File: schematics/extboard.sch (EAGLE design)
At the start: 23 parts, among them U1 LTC1257, U2 LTC1257, X1-SD SDBMF, X2-JACK 1503_02

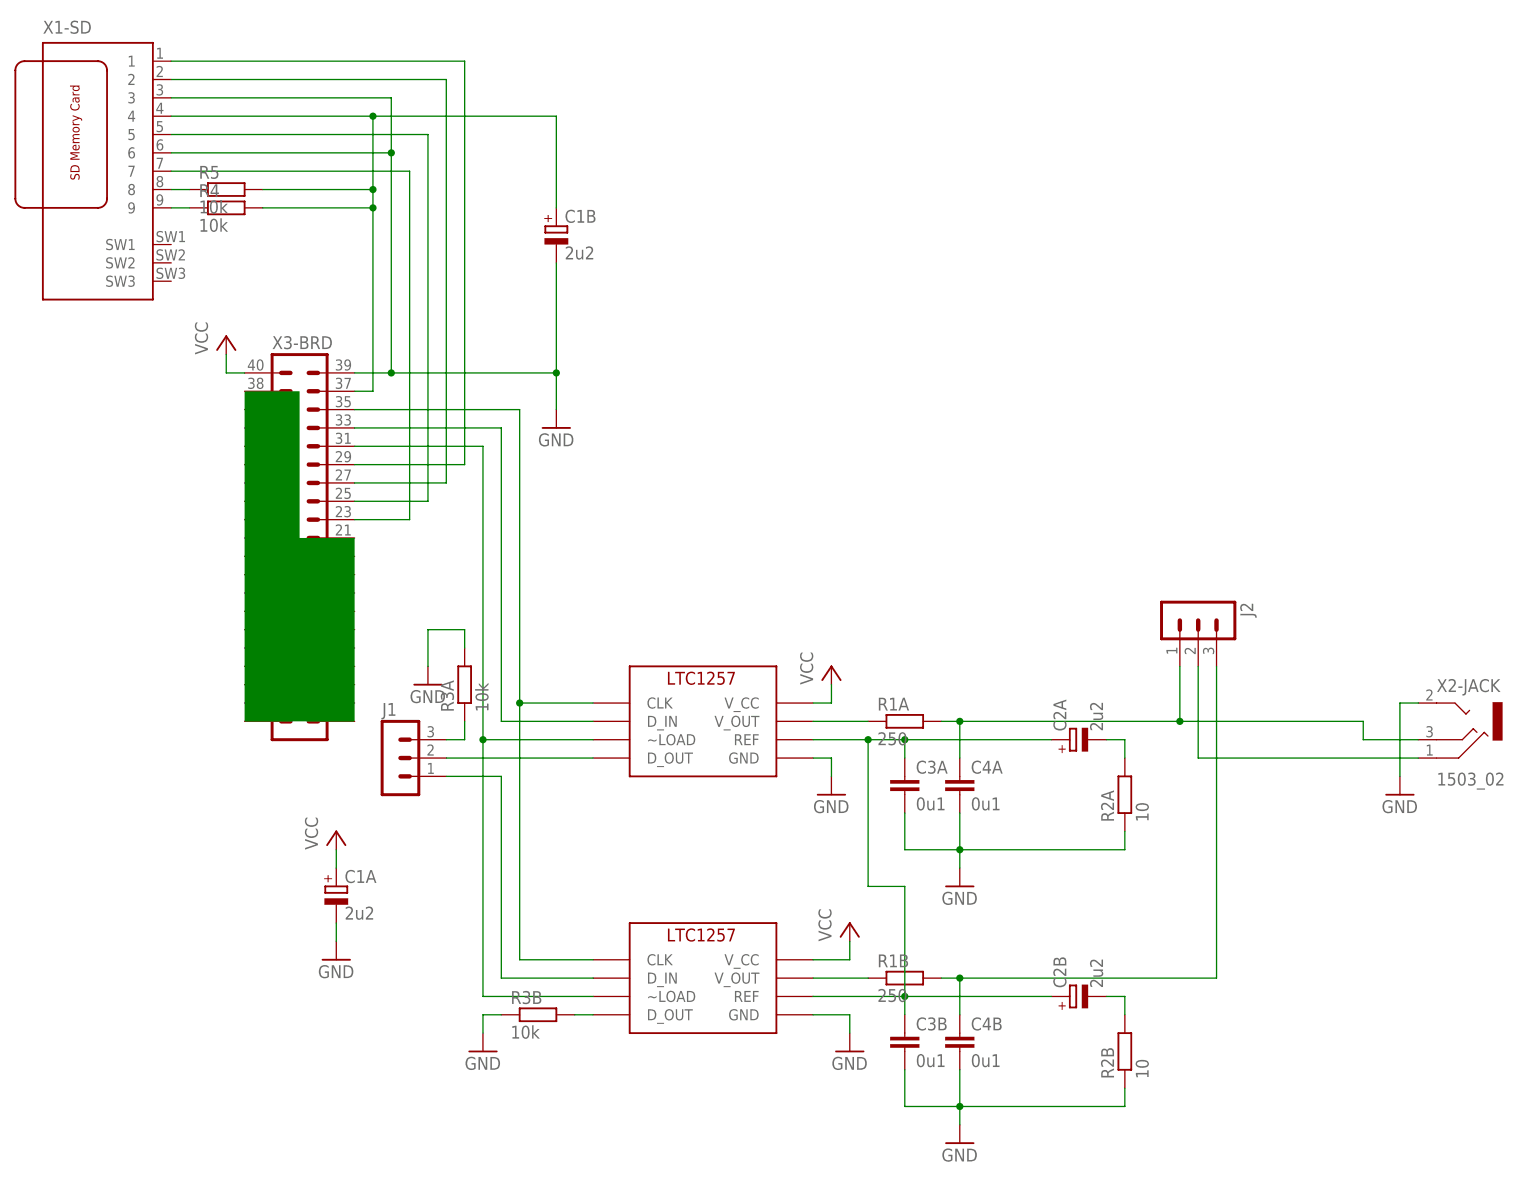
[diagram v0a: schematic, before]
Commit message: schematics: next iteration
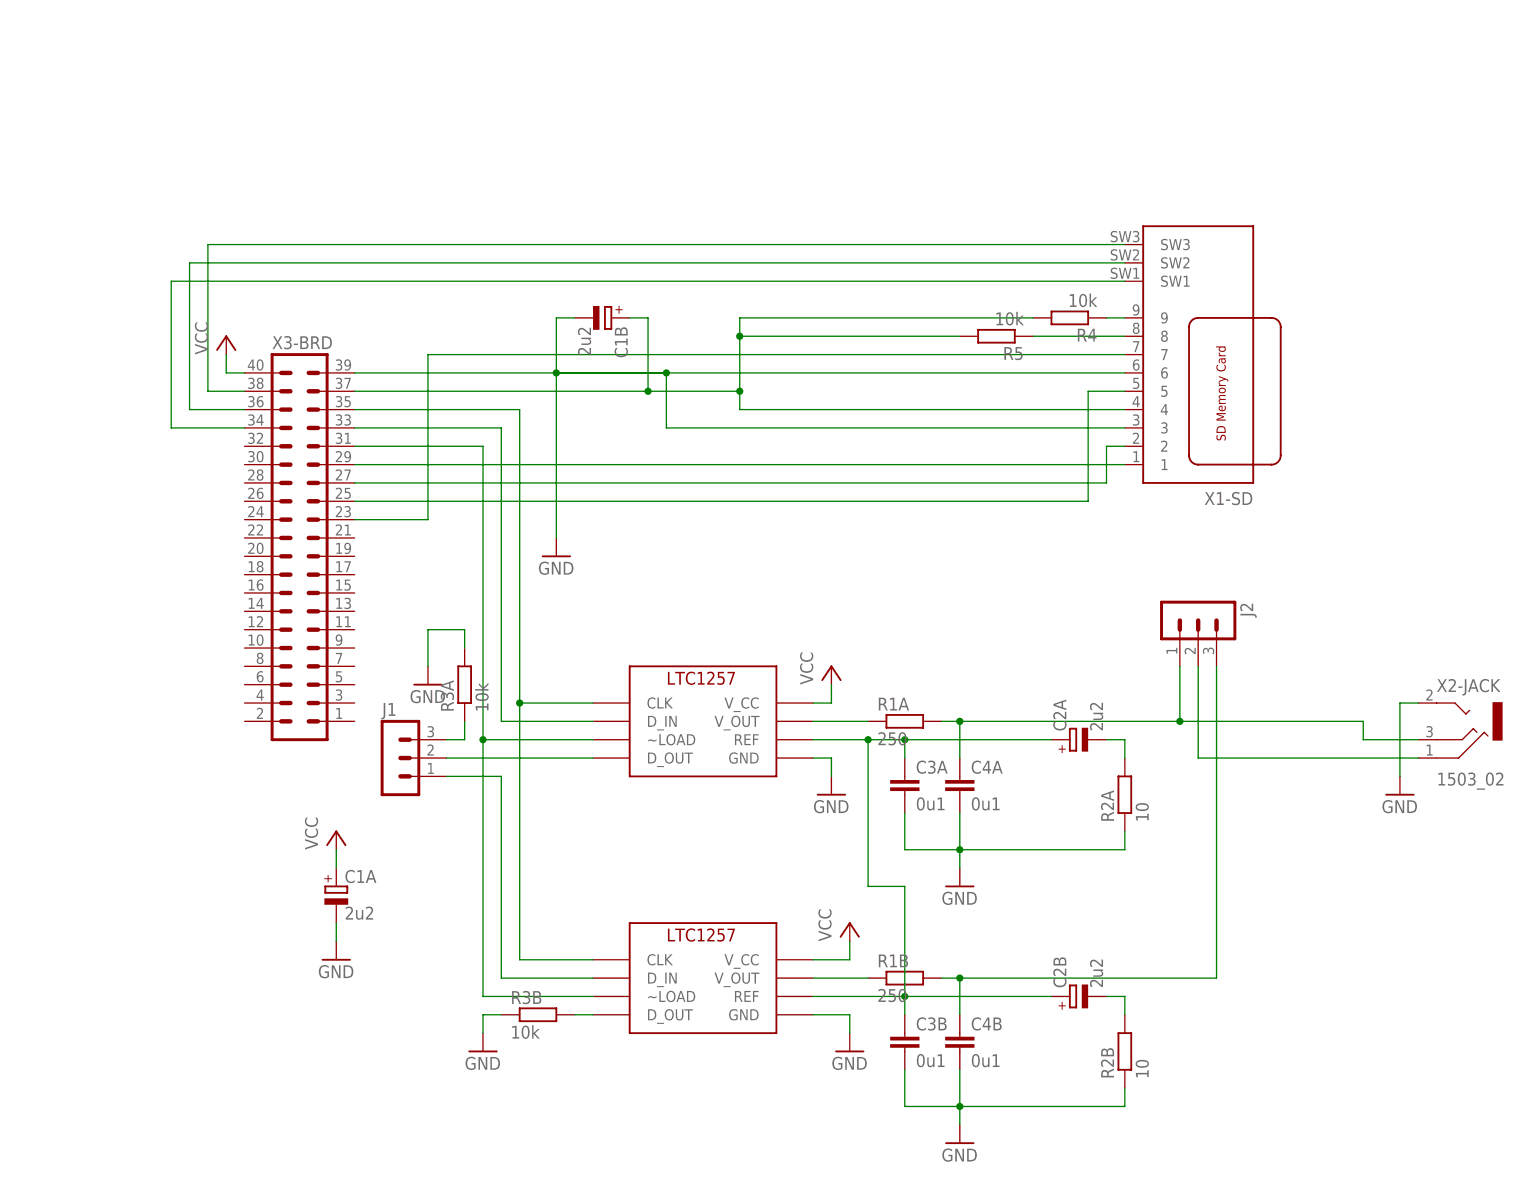
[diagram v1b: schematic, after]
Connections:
- new net N$24: X1-SD.SW1, X3-BRD.34
- new net N$25: X1-SD.SW2, X3-BRD.36
- new net N$26: X1-SD.SW3, X3-BRD.38
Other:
- moved on the sheet: C1B, R4, R5, X1-SD
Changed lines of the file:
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@@
 <sheet>
 <plain>
-<rectangle x1="-17.78" y1="17.78" x2="-10.16" y2="63.5" layer="91"/>
-<rectangle x1="-10.16" y1="17.78" x2="-2.54" y2="43.18" layer="91"/>
 </plain>
 <instances>
@@
 <instance part="R1A" gate="G$1" x="73.66" y="17.78"/>
 <instance part="R2A" gate="G$1" x="104.14" y="7.62" rot="R90"/>
-<instance part="R4" gate="G$1" x="-20.32" y="88.9"/>
-<instance part="R5" gate="G$1" x="-20.32" y="91.44"/>
+<instance part="R4" gate="G$1" x="96.52" y="73.66" rot="R180"/>
+<instance part="R5" gate="G$1" x="86.36" y="71.12" rot="R180"/>
 <instance part="R3A" gate="G$1" x="12.7" y="22.86" rot="R90"/>
 <instance part="GND2" gate="1" x="63.5" y="7.62"/>
-<instance part="GND3" gate="1" x="25.4" y="58.42"/>
+<instance part="GND3" gate="1" x="25.4" y="40.64"/>
 <instance part="GND4" gate="1" x="81.28" y="-5.08"/>
 <instance part="GND9" gate="1" x="-5.08" y="-15.24"/>
@@
 <instance part="J2" gate="G$1" x="114.3" y="33.02" rot="R270"/>
 <instance part="X2-JACK" gate="G$1" x="149.86" y="17.78"/>
-<instance part="X1-SD" gate="G$1" x="-33.02" y="91.44"/>
-<instance part="C1B" gate="G$1" x="25.4" y="86.36"/>
+<instance part="X1-SD" gate="G$1" x="109.22" y="71.12" rot="R180"/>
+<instance part="C1B" gate="G$1" x="33.02" y="73.66" rot="R270"/>
 </instances>
 <busses>
@@
 </segment>
 <segment>
+<pinref part="C1B" gate="G$1" pin="-"/>
 <pinref part="GND3" gate="1" pin="GND"/>
-<wire x1="25.4" y1="60.96" x2="25.4" y2="66.04" width="0.1524" layer="91"/>
+<wire x1="25.4" y1="43.18" x2="25.4" y2="66.04" width="0.1524" layer="91"/>
 <pinref part="X3-BRD" gate="1" pin="39"/>
-<wire x1="-2.54" y1="66.04" x2="2.54" y2="66.04" width="0.1524" layer="91"/>
-<wire x1="2.54" y1="66.04" x2="25.4" y2="66.04" width="0.1524" layer="91"/>
+<wire x1="25.4" y1="66.04" x2="25.4" y2="73.66" width="0.1524" layer="91"/>
+<wire x1="25.4" y1="73.66" x2="27.94" y2="73.66" width="0.1524" layer="91"/>
 <pinref part="X1-SD" gate="G$1" pin="3"/>
-<wire x1="2.54" y1="96.52" x2="2.54" y2="104.14" width="0.1524" layer="91"/>
-<wire x1="2.54" y1="104.14" x2="-27.94" y2="104.14" width="0.1524" layer="91"/>
+<wire x1="40.64" y1="66.04" x2="40.64" y2="58.42" width="0.1524" layer="91"/>
+<wire x1="40.64" y1="58.42" x2="104.14" y2="58.42" width="0.1524" layer="91"/>
 <pinref part="X1-SD" gate="G$1" pin="6"/>
-<wire x1="-27.94" y1="96.52" x2="2.54" y2="96.52" width="0.1524" layer="91"/>
-<junction x="2.54" y="96.52"/>
-<wire x1="2.54" y1="96.52" x2="2.54" y2="66.04" width="0.1524" layer="91"/>
-<junction x="2.54" y="66.04"/>
-<pinref part="C1B" gate="G$1" pin="-"/>
-<wire x1="25.4" y1="81.28" x2="25.4" y2="66.04" width="0.1524" layer="91"/>
+<wire x1="104.14" y1="66.04" x2="40.64" y2="66.04" width="0.1524" layer="91"/>
+<junction x="40.64" y="66.04"/>
+<wire x1="40.64" y1="66.04" x2="-2.54" y2="66.04" width="0.1524" layer="91"/>
+<wire x1="40.64" y1="66.04" x2="25.4" y2="66.04" width="0.1524" layer="91"/>
 <junction x="25.4" y="66.04"/>
 </segment>
@@
 <segment>
 <pinref part="X3-BRD" gate="1" pin="29"/>
-<wire x1="-2.54" y1="53.34" x2="12.7" y2="53.34" width="0.1524" layer="91"/>
-<wire x1="12.7" y1="53.34" x2="12.7" y2="109.22" width="0.1524" layer="91"/>
+<wire x1="-2.54" y1="53.34" x2="104.14" y2="53.34" width="0.1524" layer="91"/>
 <pinref part="X1-SD" gate="G$1" pin="1"/>
-<wire x1="-27.94" y1="109.22" x2="12.7" y2="109.22" width="0.1524" layer="91"/>
 </segment>
 </net>
@@
 <segment>
 <pinref part="X3-BRD" gate="1" pin="27"/>
-<wire x1="-2.54" y1="50.8" x2="10.16" y2="50.8" width="0.1524" layer="91"/>
-<wire x1="10.16" y1="50.8" x2="10.16" y2="106.68" width="0.1524" layer="91"/>
+<wire x1="-2.54" y1="50.8" x2="101.6" y2="50.8" width="0.1524" layer="91"/>
 <pinref part="X1-SD" gate="G$1" pin="2"/>
-<wire x1="-27.94" y1="106.68" x2="10.16" y2="106.68" width="0.1524" layer="91"/>
+<wire x1="104.14" y1="55.88" x2="101.6" y2="55.88" width="0.1524" layer="91"/>
+<wire x1="101.6" y1="55.88" x2="101.6" y2="50.8" width="0.1524" layer="91"/>
 </segment>
 </net>
@@
 <segment>
 <pinref part="X3-BRD" gate="1" pin="25"/>
-<wire x1="-2.54" y1="48.26" x2="7.62" y2="48.26" width="0.1524" layer="91"/>
-<wire x1="7.62" y1="48.26" x2="7.62" y2="99.06" width="0.1524" layer="91"/>
+<wire x1="-2.54" y1="48.26" x2="99.06" y2="48.26" width="0.1524" layer="91"/>
 <pinref part="X1-SD" gate="G$1" pin="5"/>
-<wire x1="-27.94" y1="99.06" x2="7.62" y2="99.06" width="0.1524" layer="91"/>
+<wire x1="104.14" y1="63.5" x2="99.06" y2="63.5" width="0.1524" layer="91"/>
+<wire x1="99.06" y1="63.5" x2="99.06" y2="48.26" width="0.1524" layer="91"/>
 </segment>
 </net>
@@
 <segment>
 <pinref part="X3-BRD" gate="1" pin="23"/>
-<wire x1="-2.54" y1="45.72" x2="5.08" y2="45.72" width="0.1524" layer="91"/>
-<wire x1="5.08" y1="45.72" x2="5.08" y2="93.98" width="0.1524" layer="91"/>
+<wire x1="-2.54" y1="45.72" x2="7.62" y2="45.72" width="0.1524" layer="91"/>
+<wire x1="7.62" y1="45.72" x2="7.62" y2="68.58" width="0.1524" layer="91"/>
 <pinref part="X1-SD" gate="G$1" pin="7"/>
-<wire x1="5.08" y1="93.98" x2="-27.94" y2="93.98" width="0.1524" layer="91"/>
+<wire x1="7.62" y1="68.58" x2="104.14" y2="68.58" width="0.1524" layer="91"/>
 </segment>
 </net>
@@
 <pinref part="X1-SD" gate="G$1" pin="8"/>
 <pinref part="R5" gate="G$1" pin="1"/>
-<wire x1="-27.94" y1="91.44" x2="-25.4" y2="91.44" width="0.1524" layer="91"/>
+<wire x1="104.14" y1="71.12" x2="91.44" y2="71.12" width="0.1524" layer="91"/>
 </segment>
 </net>
@@
 <pinref part="X1-SD" gate="G$1" pin="9"/>
 <pinref part="R4" gate="G$1" pin="1"/>
-<wire x1="-27.94" y1="88.9" x2="-25.4" y2="88.9" width="0.1524" layer="91"/>
+<wire x1="104.14" y1="73.66" x2="101.6" y2="73.66" width="0.1524" layer="91"/>
 </segment>
 </net>
 <net name="N$11" class="0">
 <segment>
+<pinref part="R5" gate="G$1" pin="2"/>
+<pinref part="C1B" gate="G$1" pin="+"/>
+<wire x1="38.1" y1="73.66" x2="35.56" y2="73.66" width="0.1524" layer="91"/>
 <pinref part="X3-BRD" gate="1" pin="37"/>
-<wire x1="-2.54" y1="63.5" x2="0" y2="63.5" width="0.1524" layer="91"/>
+<wire x1="50.8" y1="63.5" x2="38.1" y2="63.5" width="0.1524" layer="91"/>
+<wire x1="38.1" y1="63.5" x2="-2.54" y2="63.5" width="0.1524" layer="91"/>
+<wire x1="38.1" y1="73.66" x2="38.1" y2="63.5" width="0.1524" layer="91"/>
+<junction x="38.1" y="63.5"/>
+<wire x1="50.8" y1="63.5" x2="50.8" y2="60.96" width="0.1524" layer="91"/>
 <pinref part="X1-SD" gate="G$1" pin="4"/>
-<wire x1="-27.94" y1="101.6" x2="0" y2="101.6" width="0.1524" layer="91"/>
-<wire x1="0" y1="101.6" x2="0" y2="91.44" width="0.1524" layer="91"/>
-<pinref part="R5" gate="G$1" pin="2"/>
-<wire x1="0" y1="91.44" x2="0" y2="88.9" width="0.1524" layer="91"/>
-<wire x1="0" y1="88.9" x2="0" y2="63.5" width="0.1524" layer="91"/>
-<wire x1="-15.24" y1="91.44" x2="0" y2="91.44" width="0.1524" layer="91"/>
-<junction x="0" y="91.44"/>
+<wire x1="104.14" y1="60.96" x2="50.8" y2="60.96" width="0.1524" layer="91"/>
+<wire x1="50.8" y1="63.5" x2="50.8" y2="71.12" width="0.1524" layer="91"/>
+<junction x="50.8" y="63.5"/>
+<wire x1="81.28" y1="71.12" x2="50.8" y2="71.12" width="0.1524" layer="91"/>
+<wire x1="50.8" y1="71.12" x2="50.8" y2="73.66" width="0.1524" layer="91"/>
+<junction x="50.8" y="71.12"/>
 <pinref part="R4" gate="G$1" pin="2"/>
-<wire x1="0" y1="88.9" x2="-15.24" y2="88.9" width="0.1524" layer="91"/>
-<junction x="0" y="88.9"/>
-<pinref part="C1B" gate="G$1" pin="+"/>
-<wire x1="0" y1="101.6" x2="25.4" y2="101.6" width="0.1524" layer="91"/>
-<wire x1="25.4" y1="101.6" x2="25.4" y2="88.9" width="0.1524" layer="91"/>
-<junction x="0" y="101.6"/>
-</segment>
-</net>
+<wire x1="50.8" y1="73.66" x2="91.44" y2="73.66" width="0.1524" layer="91"/>
+</segment>
+</net>
+<net name="N$24" class="0">
+<segment>
+<pinref part="X1-SD" gate="G$1" pin="SW1"/>
+<wire x1="-27.94" y1="78.74" x2="104.14" y2="78.74" width="0.1524" layer="91"/>
+<pinref part="X3-BRD" gate="1" pin="34"/>
+<wire x1="-17.78" y1="58.42" x2="-27.94" y2="58.42" width="0.1524" layer="91"/>
+<wire x1="-27.94" y1="58.42" x2="-27.94" y2="78.74" width="0.1524" layer="91"/>
+</segment>
+</net>
+<net name="N$25" class="0">
+<segment>
+<pinref part="X1-SD" gate="G$1" pin="SW2"/>
+<wire x1="104.14" y1="81.28" x2="-25.4" y2="81.28" width="0.1524" layer="91"/>
+<wire x1="-25.4" y1="81.28" x2="-25.4" y2="60.96" width="0.1524" layer="91"/>
+<pinref part="X3-BRD" gate="1" pin="36"/>
+<wire x1="-25.4" y1="60.96" x2="-17.78" y2="60.96" width="0.1524" layer="91"/>
+</segment>
+</net>
+<net name="N$26" class="0">
+<segment>
+<pinref part="X1-SD" gate="G$1" pin="SW3"/>
+<wire x1="-22.86" y1="83.82" x2="104.14" y2="83.82" width="0.1524" layer="91"/>
+<wire x1="-22.86" y1="83.82" x2="-22.86" y2="63.5" width="0.1524" layer="91"/>
+<pinref part="X3-BRD" gate="1" pin="38"/>
+<wire x1="-22.86" y1="63.5" x2="-17.78" y2="63.5" width="0.1524" layer="91"/>
+</segment>
+</net>
